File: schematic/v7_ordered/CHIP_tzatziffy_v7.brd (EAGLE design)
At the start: 40.9 x 49.8 mm, 60 parts, among them J1 2X20-CHIP0.7_DRILL, Q2 n.a. / 2N7002ET1G, U1 n.a. / LMR62421, U3 DS2431P, X1 FH12-40S-0.5SH

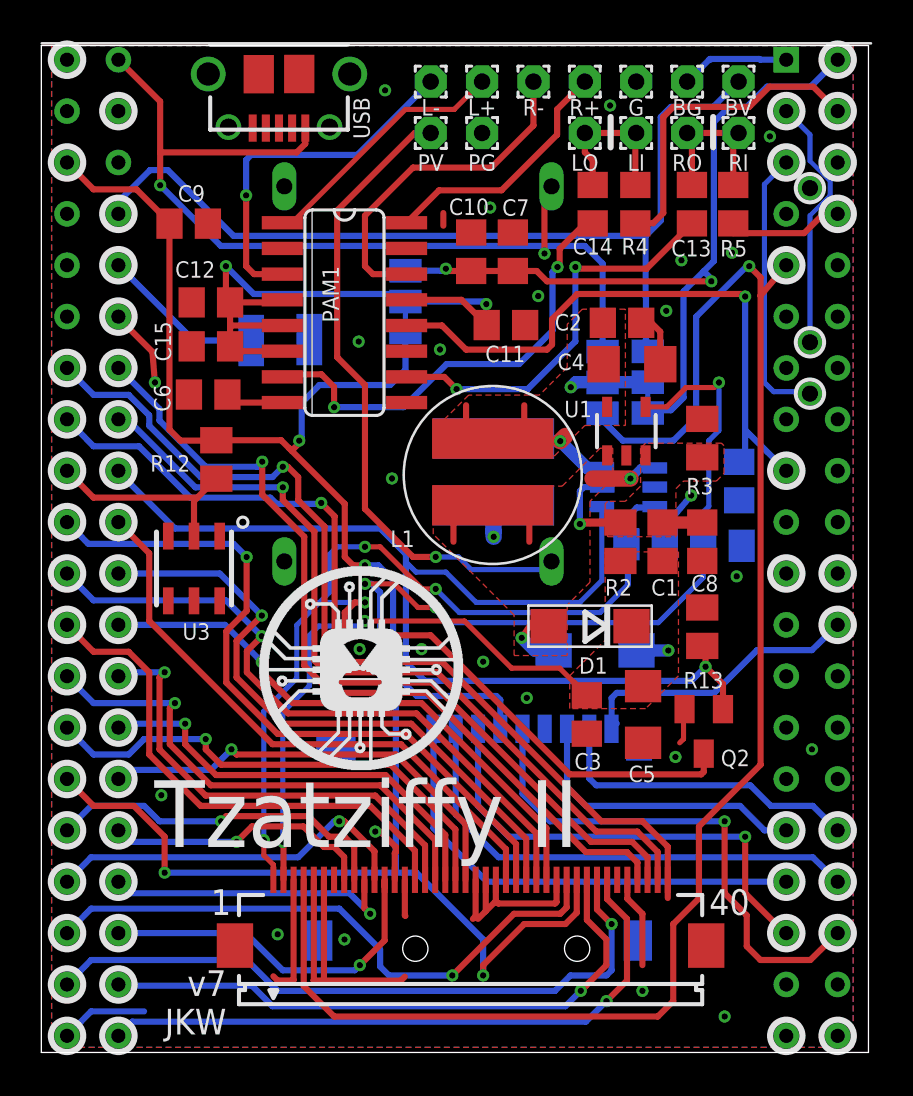
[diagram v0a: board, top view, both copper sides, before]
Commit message: moved to ordered
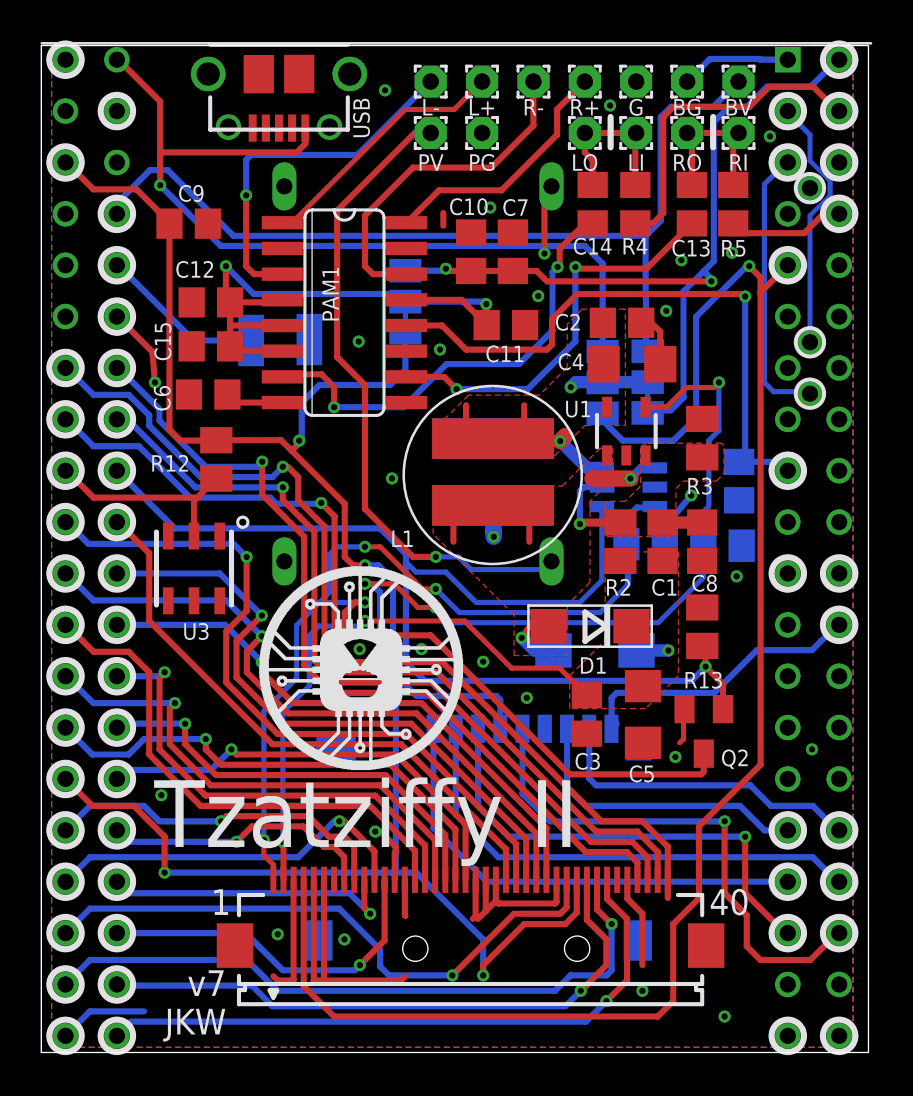
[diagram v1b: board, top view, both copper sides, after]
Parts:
- J1: value 2X20-CHIP0.7_DRILL -> 2X20-CHIP0.8_DRILL_0.15OFFSET_LR; device JKW_CHIP:2X20CHIP_NOOFFSET-TH_0.7 -> JKW_CHIP:2X20CHIP_0.15MM_OFFSET_TH_08
